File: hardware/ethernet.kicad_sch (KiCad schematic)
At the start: 39 parts, among them J1 RJ45_Hanrun_HR911105A_Horizon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, U1 W5500, Y1 25MHz

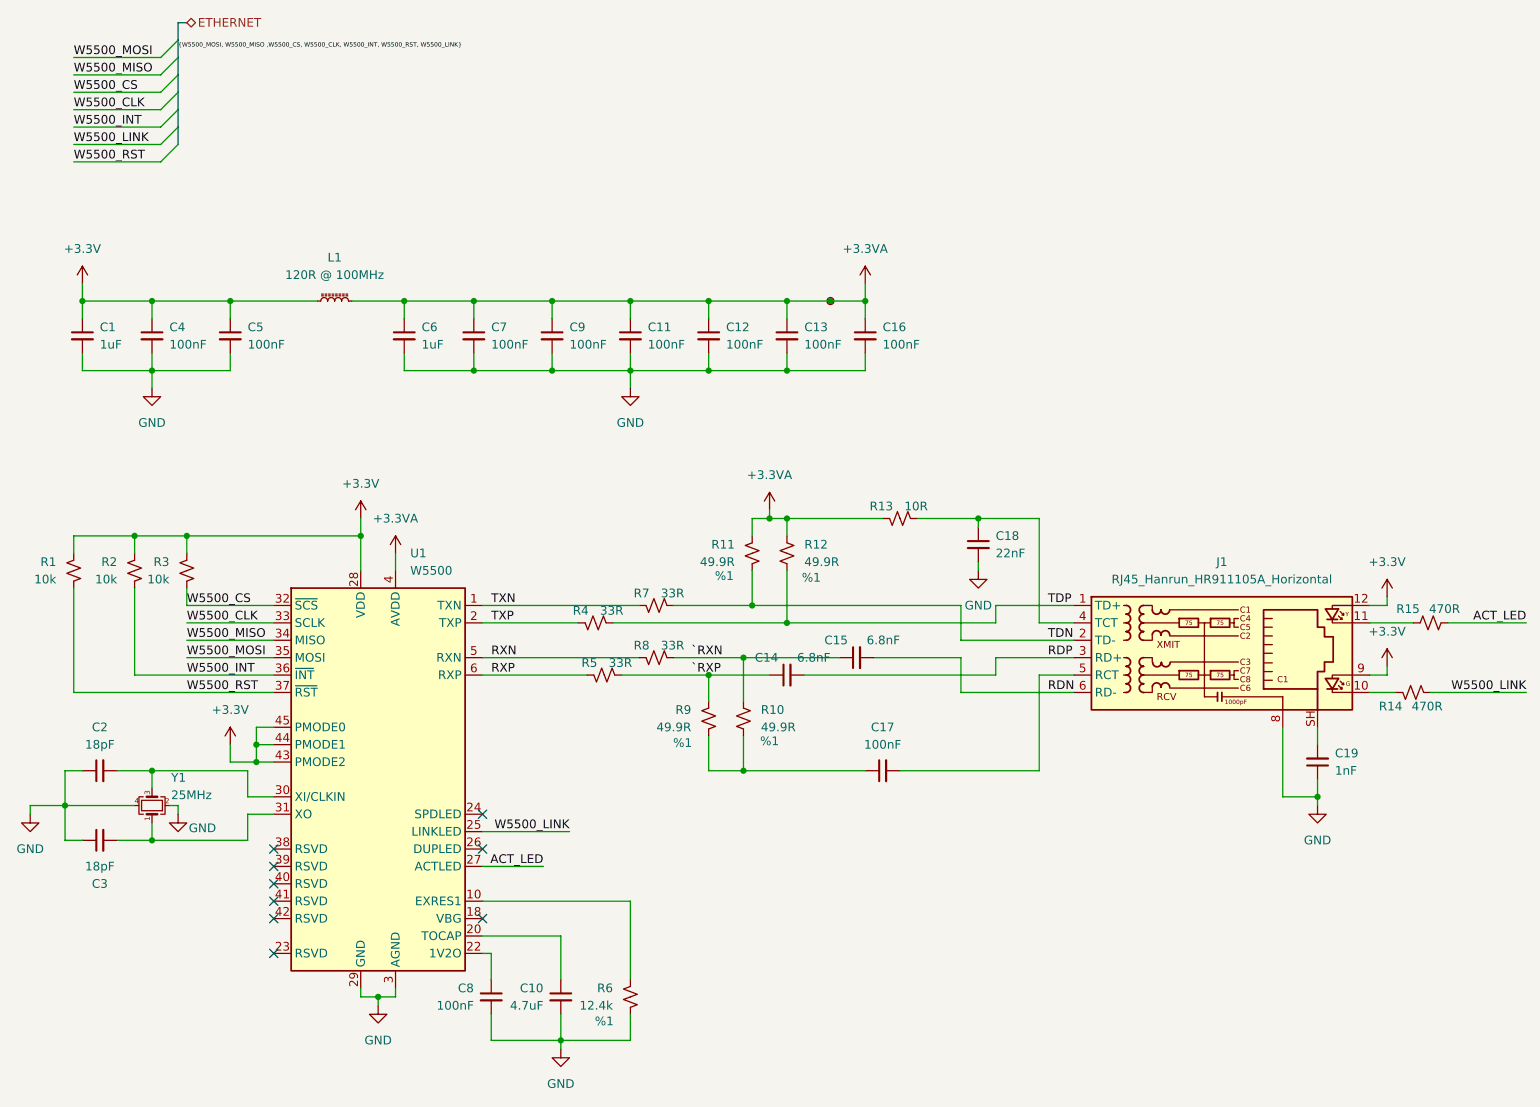
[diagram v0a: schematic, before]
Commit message: Added Board Register
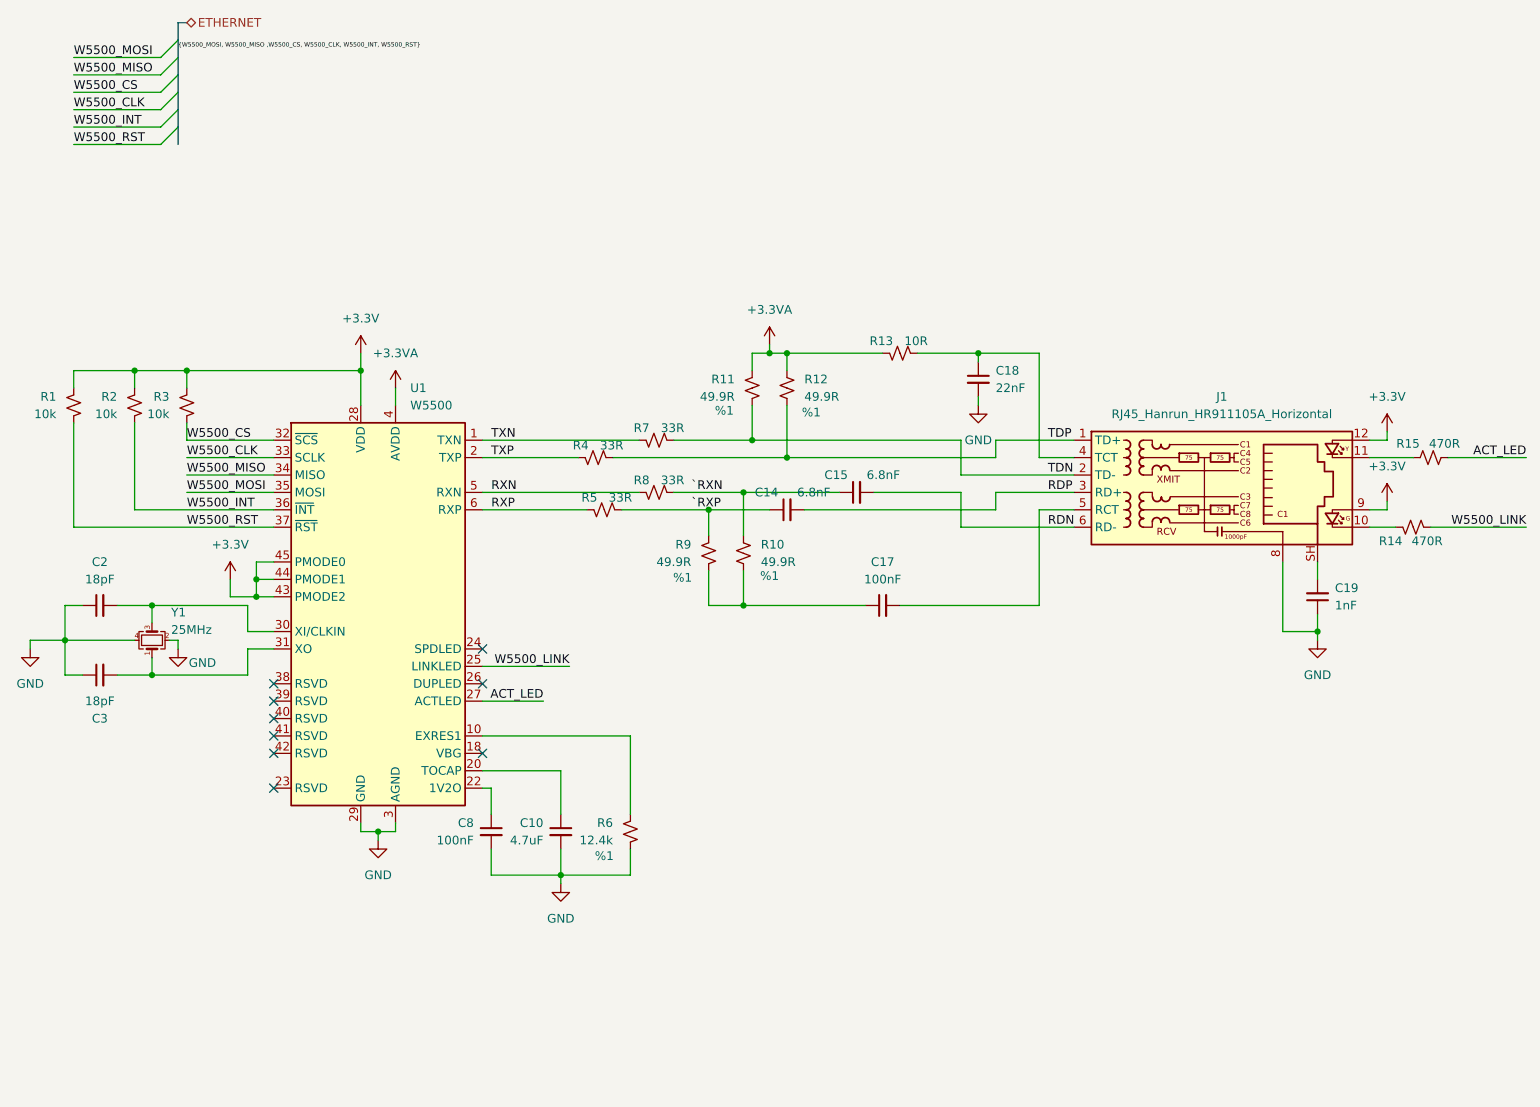
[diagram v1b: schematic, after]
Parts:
- removed C1, C6: 1uF, Capacitor_SMD:C_0603_1608Metric, symbol Device:C_Small
- removed C11, C12, C13, C16, C4, C5, C7, C9: 100nF, Capacitor_SMD:C_0603_1608Metric, symbol Device:C_Small
- removed L1: 120R @ 100MHz, Inductor_SMD:L_0603_1608Metric, symbol Device:L_Ferrite_Small
- removed TP1: TestPoint_Small, TestPoint:TestPoint_Pad_D1.5mm, symbol Connector:TestPoint_Small
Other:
- moved on the sheet: C10, C14, C15, C17, C18, C19, C2, C3, C8, J1, R1, R10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
